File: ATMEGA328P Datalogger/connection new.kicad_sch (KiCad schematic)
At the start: 4 parts, among them J1 Conn_01x04_Pin, J2 Conn_01x04_Pin, J3 Conn_01x09_Pin, J4 Conn_02x03_Odd_Even

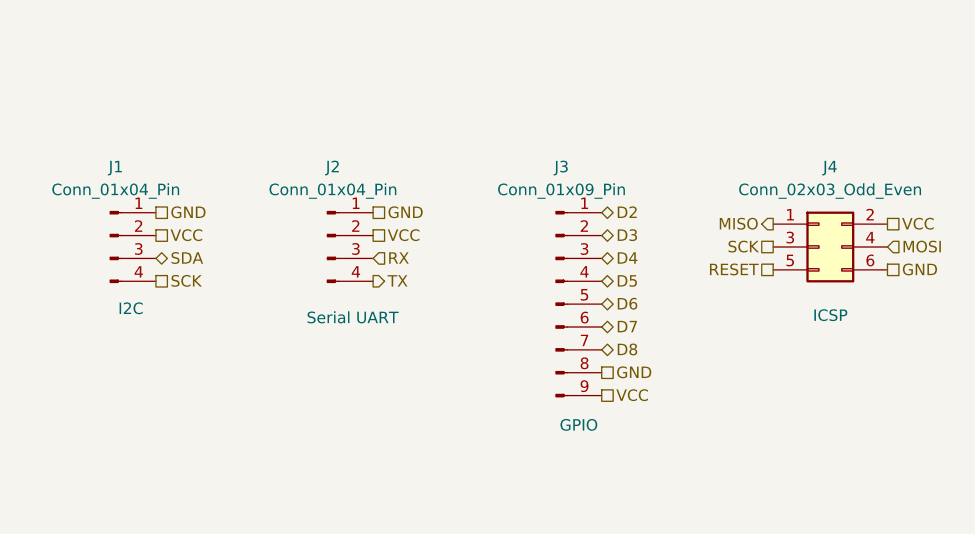
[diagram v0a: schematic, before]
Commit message: Finally all bugs settled
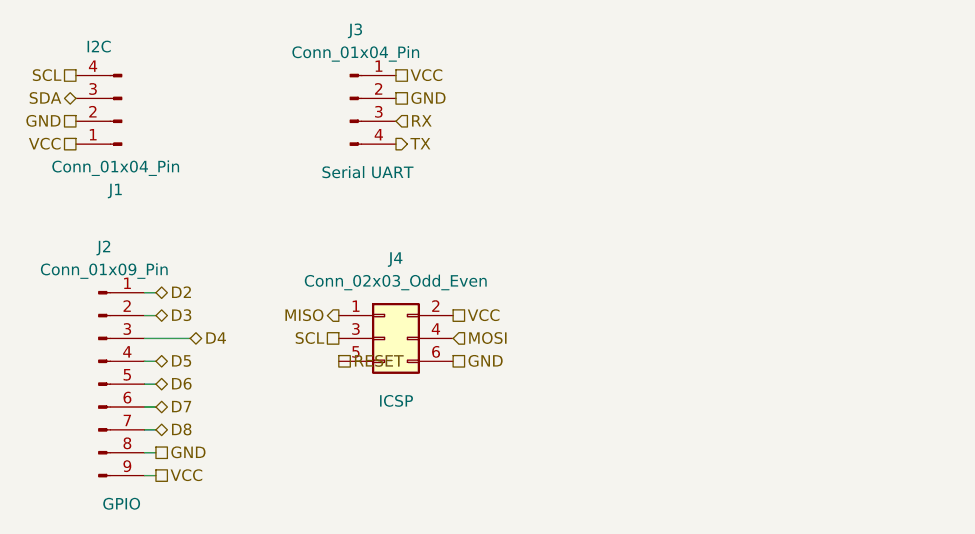
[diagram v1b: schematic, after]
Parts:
- removed J2: Conn_01x04_Pin, Connector_PinSocket_2.54mm:PinSocket_1x04_P2.54mm_Vertical, symbol Connector:Conn_01x04_Pin
- removed J3: Conn_01x09_Pin, Connector_PinSocket_2.54mm:PinSocket_1x09_P2.54mm_Vertical, symbol Connector:Conn_01x09_Pin
- added J2: Conn_01x09_Pin, symbol Connector:Conn_01x09_Pin
- added J3: Conn_01x04_Pin, symbol Connector:Conn_01x04_Pin
- J1: footprint Connector_PinSocket_2.54mm:PinSocket_1x04_P2.54mm_Vertical -> (none)
- J4: footprint Connector_PinSocket_2.54mm:PinSocket_2x03_P2.54mm_Vertical -> (none)
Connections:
- net D2: now also J2.1 (Pin_1)
- net D3: now also J2.2 (Pin_2)
- net D4: now also J2.3 (Pin_3)
- net D5: now also J2.4 (Pin_4)
- net D6: now also J2.5 (Pin_5)
- net D7: now also J2.6 (Pin_6)
- net D8: now also J2.7 (Pin_7)
- net GND: now also J1.2 (Pin_2), J2.8 (Pin_8), J3.2 (Pin_2); no longer J1.1 (Pin_1)
- net RX: now also J3.3 (Pin_3)
- net TX: now also J3.4 (Pin_4)
- net VCC: now also J1.1 (Pin_1), J2.9 (Pin_9), J3.1 (Pin_1); no longer J1.2 (Pin_2)
- net SCK renamed SCL
